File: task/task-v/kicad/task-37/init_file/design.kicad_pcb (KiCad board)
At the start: 2 copper layers, 140 x 110 mm, 8 parts, among them U1 ANT, U2 LNA, U3 BPF, U4 MIX, U5 AMP, U6 LPF, U7 ADC, U8 DAQ

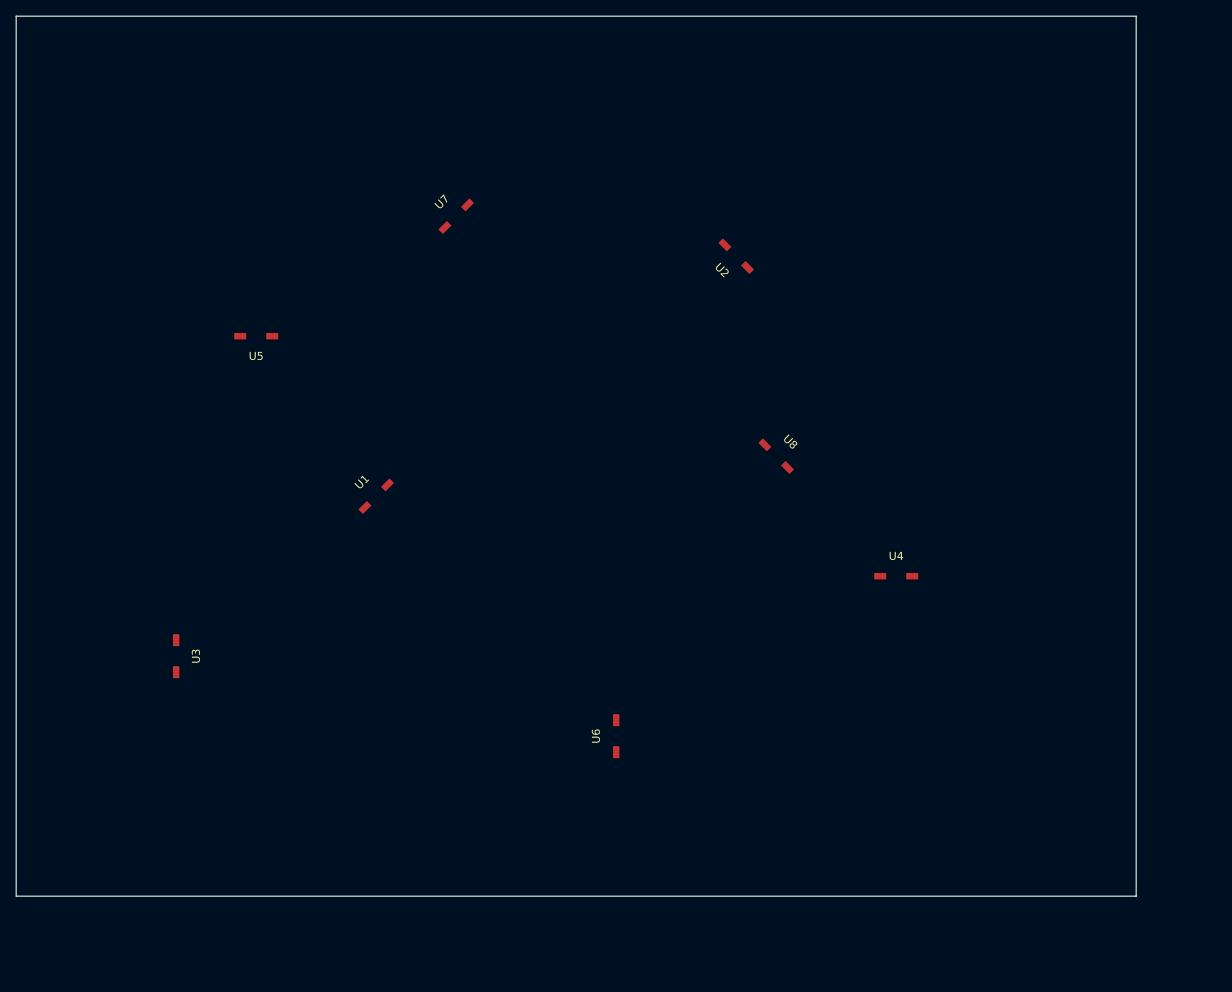
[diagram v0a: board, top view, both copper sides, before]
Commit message: Refine engineering task metadata and instructions
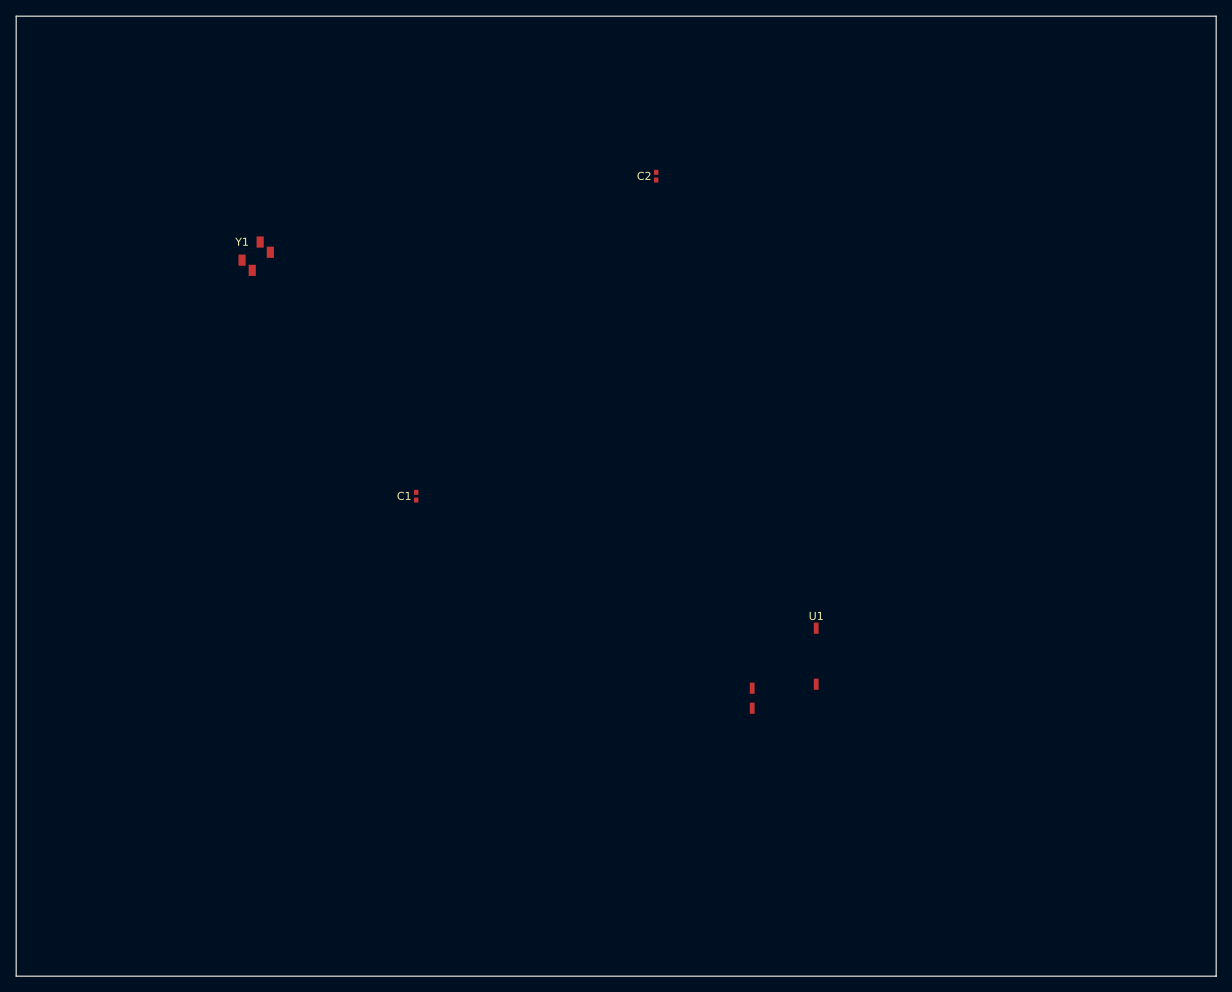
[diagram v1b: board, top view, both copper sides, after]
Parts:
- removed U2: LNA, Package_SO:SOIC-8_3.9x4.9mm_P1.27mm
- removed U3: BPF, Package_SO:SOIC-8_3.9x4.9mm_P1.27mm
- removed U4: MIX, Package_SO:SOIC-8_3.9x4.9mm_P1.27mm
- removed U5: AMP, Package_SO:SOIC-8_3.9x4.9mm_P1.27mm
- removed U6: LPF, Package_SO:SOIC-8_3.9x4.9mm_P1.27mm
- removed U7: ADC, Package_SO:SOIC-16_3.9x9.9mm_P1.27mm
- removed U8: DAQ, Package_SO:SOIC-16_3.9x9.9mm_P1.27mm
- added C1: 12pF, Capacitor_SMD:C_0402_1005Metric, F.Cu at (50.0, 60.0)
- added C2: 12pF, Capacitor_SMD:C_0402_1005Metric, F.Cu at (80.0, 20.0)
- added Y1: 8MHz, Crystal:Crystal_SMD_3225-4Pin_3.2x2.5mm, F.Cu at (30.0, 30.0)
- U1: value ANT -> STM32F103; footprint Connector_Coaxial:SMA_Amphenol_901-143-8RFX_Vertical -> Package_QFP:LQFP-48_7x7mm_P0.5mm
- moved U1 58.5 mm to (100.0, 80.0), turned to 0 degrees
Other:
- board size 140 x 110 mm -> 150 x 120 mm
- copper layers 2 -> 3
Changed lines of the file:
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@@
   (layers
     (0 "F.Cu" signal)
+    (1 "In1.Cu" power)
     (31 "B.Cu" signal)
     (36 "B.Paste" user)
@@
     (pad_to_mask_clearance 0)
   )
-  (gr_rect (start 0 0) (end 140 110) (layer "Edge.Cuts") (width 0.05))
-  (footprint "Connector_Coaxial:SMA_Amphenol_901-143-8RFX_Vertical"
+  (gr_rect (start 0 0) (end 150 120) (layer "Edge.Cuts") (width 0.05))
+  (footprint "Package_QFP:LQFP-48_7x7mm_P0.5mm"
     (layer "F.Cu")
-    (at 45.000 60.000 45)
-    (fp_text reference "U1" (at 0 -2.5 45) (layer "F.SilkS")
+    (at 100.000 80.000 0)
+    (fp_text reference "U1" (at 0 -5) (layer "F.SilkS")
       (effects (font (size 1 1) (thickness 0.15)))
     )
-    (fp_text value "ANT" (at 0 2.5 45) (layer "F.Fab")
+    (fp_text value "STM32F103" (at 0 5) (layer "F.Fab")
       (effects (font (size 1 1) (thickness 0.15)))
     )
-    (pad "1" smd rect (at -2 0 45) (size 1.5 0.8) (layers "F.Cu" "F.Paste" "F.Mask"))
-    (pad "2" smd rect (at 2 0 45) (size 1.5 0.8) (layers "F.Cu" "F.Paste" "F.Mask"))
+    (pad "OSC_IN" smd rect (at -8.000 4.000) (size 0.6 1.4) (layers "F.Cu" "F.Paste" "F.Mask"))
+    (pad "OSC_OUT" smd rect (at -8.000 6.500) (size 0.6 1.4) (layers "F.Cu" "F.Paste" "F.Mask"))
+    (pad "GND" smd rect (at 0 -3.5) (size 0.6 1.4) (layers "F.Cu" "F.Paste" "F.Mask"))
+    (pad "VDD" smd rect (at 0 3.5) (size 0.6 1.4) (layers "F.Cu" "F.Paste" "F.Mask"))
   )
-  (footprint "Package_SO:SOIC-8_3.9x4.9mm_P1.27mm"
+  (footprint "Crystal:Crystal_SMD_3225-4Pin_3.2x2.5mm"
     (layer "F.Cu")
-    (at 90.000 30.000 135)
-    (fp_text reference "U2" (at 0 -2.5 135) (layer "F.SilkS")
+    (at 30.000 30.000 45)
+    (fp_text reference "Y1" (at 0 -2.5) (layer "F.SilkS")
       (effects (font (size 1 1) (thickness 0.15)))
     )
-    (fp_text value "LNA" (at 0 2.5 135) (layer "F.Fab")
+    (fp_text value "8MHz" (at 0 2.5) (layer "F.Fab")
       (effects (font (size 1 1) (thickness 0.15)))
     )
-    (pad "1" smd rect (at -2 0 135) (size 1.5 0.8) (layers "F.Cu" "F.Paste" "F.Mask"))
-    (pad "2" smd rect (at 2 0 135) (size 1.5 0.8) (layers "F.Cu" "F.Paste" "F.Mask"))
+    (pad "1" smd rect (at -1.6 0.9) (size 0.9 1.4) (layers "F.Cu" "F.Paste" "F.Mask"))
+    (pad "2" smd rect (at 1.6 0.9) (size 0.9 1.4) (layers "F.Cu" "F.Paste" "F.Mask"))
+    (pad "3" smd rect (at 1.6 -0.9) (size 0.9 1.4) (layers "F.Cu" "F.Paste" "F.Mask"))
+    (pad "4" smd rect (at -1.6 -0.9) (size 0.9 1.4) (layers "F.Cu" "F.Paste" "F.Mask"))
   )
-  (footprint "Package_SO:SOIC-8_3.9x4.9mm_P1.27mm"
+  (footprint "Capacitor_SMD:C_0402_1005Metric"
     (layer "F.Cu")
-    (at 20.000 80.000 270)
-    (fp_text reference "U3" (at 0 -2.5 270) (layer "F.SilkS")
+    (at 50.000 60.000 90)
+    (fp_text reference "C1" (at 0 -1.5) (layer "F.SilkS")
       (effects (font (size 1 1) (thickness 0.15)))
     )
-    (fp_text value "BPF" (at 0 2.5 270) (layer "F.Fab")
+    (fp_text value "12pF" (at 0 1.5) (layer "F.Fab")
       (effects (font (size 1 1) (thickness 0.15)))
     )
-    (pad "1" smd rect (at -2 0 270) (size 1.5 0.8) (layers "F.Cu" "F.Paste" "F.Mask"))
-    (pad "2" smd rect (at 2 0 270) (size 1.5 0.8) (layers "F.Cu" "F.Paste" "F.Mask"))
+    (pad "1" smd rect (at -0.48 0) (size 0.56 0.62) (layers "F.Cu" "F.Paste" "F.Mask"))
+    (pad "2" smd rect (at 0.48 0) (size 0.56 0.62) (layers "F.Cu" "F.Paste" "F.Mask"))
   )
-  (footprint "Package_SO:SOIC-8_3.9x4.9mm_P1.27mm"
+  (footprint "Capacitor_SMD:C_0402_1005Metric"
     (layer "F.Cu")
-    (at 110.000 70.000 0)
-    (fp_text reference "U4" (at 0 -2.5 0) (layer "F.SilkS")
+    (at 80.000 20.000 90)
+    (fp_text reference "C2" (at 0 -1.5) (layer "F.SilkS")
       (effects (font (size 1 1) (thickness 0.15)))
     )
-    (fp_text value "MIX" (at 0 2.5 0) (layer "F.Fab")
+    (fp_text value "12pF" (at 0 1.5) (layer "F.Fab")
       (effects (font (size 1 1) (thickness 0.15)))
     )
-    (pad "1" smd rect (at -2 0 0) (size 1.5 0.8) (layers "F.Cu" "F.Paste" "F.Mask"))
-    (pad "2" smd rect (at 2 0 0) (size 1.5 0.8) (layers "F.Cu" "F.Paste" "F.Mask"))
-  )
-  (footprint "Package_SO:SOIC-8_3.9x4.9mm_P1.27mm"
-    (layer "F.Cu")
-    (at 30.000 40.000 180)
-    (fp_text reference "U5" (at 0 -2.5 180) (layer "F.SilkS")
-      (effects (font (size 1 1) (thickness 0.15)))
-    )
-    (fp_text value "AMP" (at 0 2.5 180) (layer "F.Fab")
-      (effects (font (size 1 1) (thickness 0.15)))
-    )
-    (pad "1" smd rect (at -2 0 180) (size 1.5 0.8) (layers "F.Cu" "F.Paste" "F.Mask"))
-    (pad "2" smd rect (at 2 0 180) (size 1.5 0.8) (layers "F.Cu" "F.Paste" "F.Mask"))
-  )
-  (footprint "Package_SO:SOIC-8_3.9x4.9mm_P1.27mm"
-    (layer "F.Cu")
-    (at 75.000 90.000 90)
-    (fp_text reference "U6" (at 0 -2.5 90) (layer "F.SilkS")
-      (effects (font (size 1 1) (thickness 0.15)))
-    )
-    (fp_text value "LPF" (at 0 2.5 90) (layer "F.Fab")
-      (effects (font (size 1 1) (thickness 0.15)))
-    )
-    (pad "1" smd rect (at -2 0 90) (size 1.5 0.8) (layers "F.Cu" "F.Paste" "F.Mask"))
-    (pad "2" smd rect (at 2 0 90) (size 1.5 0.8) (layers "F.Cu" "F.Paste" "F.Mask"))
-  )
-  (footprint "Package_SO:SOIC-16_3.9x9.9mm_P1.27mm"
-    (layer "F.Cu")
-    (at 55.000 25.000 45)
-    (fp_text reference "U7" (at 0 -2.5 45) (layer "F.SilkS")
-      (effects (font (size 1 1) (thickness 0.15)))
-    )
-    (fp_text value "ADC" (at 0 2.5 45) (layer "F.Fab")
-      (effects (font (size 1 1) (thickness 0.15)))
-    )
-    (pad "1" smd rect (at -2 0 45) (size 1.5 0.8) (layers "F.Cu" "F.Paste" "F.Mask"))
-    (pad "2" smd rect (at 2 0 45) (size 1.5 0.8) (layers "F.Cu" "F.Paste" "F.Mask"))
-  )
-  (footprint "Package_SO:SOIC-16_3.9x9.9mm_P1.27mm"
-    (layer "F.Cu")
-    (at 95.000 55.000 315)
-    (fp_text reference "U8" (at 0 -2.5 315) (layer "F.SilkS")
-      (effects (font (size 1 1) (thickness 0.15)))
-    )
-    (fp_text value "DAQ" (at 0 2.5 315) (layer "F.Fab")
-      (effects (font (size 1 1) (thickness 0.15)))
-    )
-    (pad "1" smd rect (at -2 0 315) (size 1.5 0.8) (layers "F.Cu" "F.Paste" "F.Mask"))
-    (pad "2" smd rect (at 2 0 315) (size 1.5 0.8) (layers "F.Cu" "F.Paste" "F.Mask"))
+    (pad "1" smd rect (at -0.48 0) (size 0.56 0.62) (layers "F.Cu" "F.Paste" "F.Mask"))
+    (pad "2" smd rect (at 0.48 0) (size 0.56 0.62) (layers "F.Cu" "F.Paste" "F.Mask"))
   )
 )
